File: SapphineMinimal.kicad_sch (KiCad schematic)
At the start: 6 parts

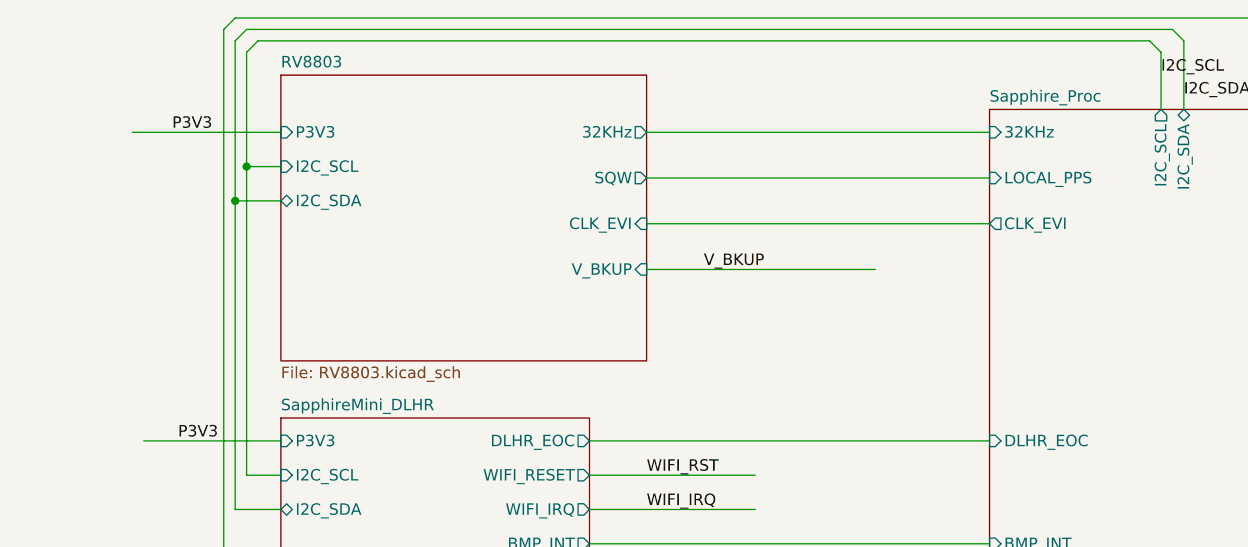
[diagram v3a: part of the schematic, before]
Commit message: End of Weekend
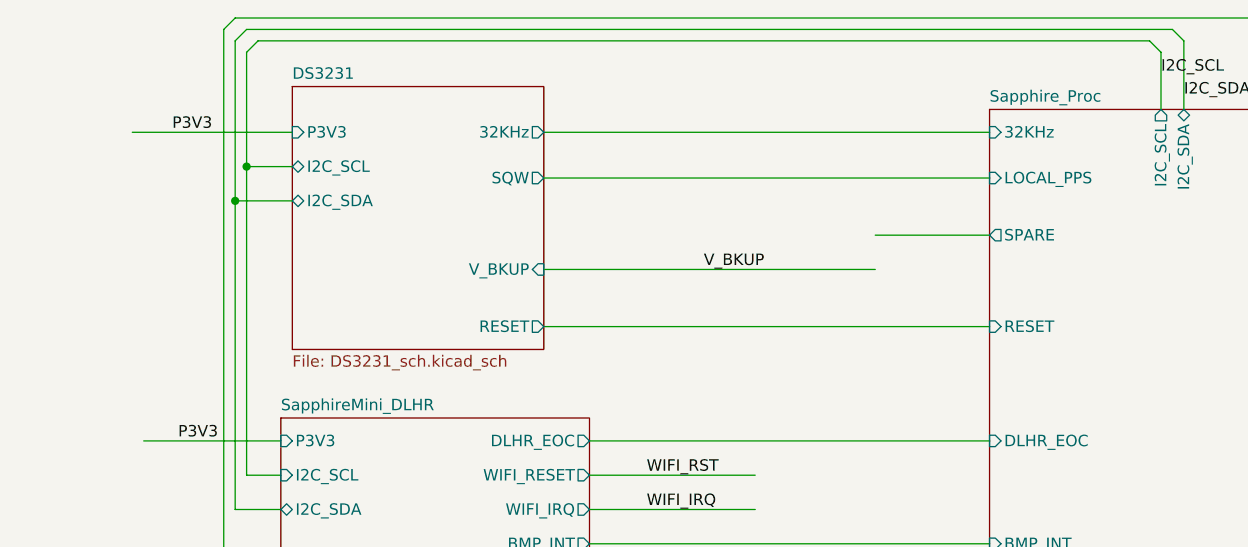
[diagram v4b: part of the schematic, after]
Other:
- removed sheet RV8803
- added sheet DS3231 (DS3231_sch.kicad_sch)
- sheet Sapphire_Proc ports: added RESET, SPARE; removed CLK_EVI
